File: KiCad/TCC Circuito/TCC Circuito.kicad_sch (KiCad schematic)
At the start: 6 parts, among them J1 Sensor HALL, J2 Rasp pico, U1 TL071, U2 INA333xxDGK, U3 ADS1115IDGS

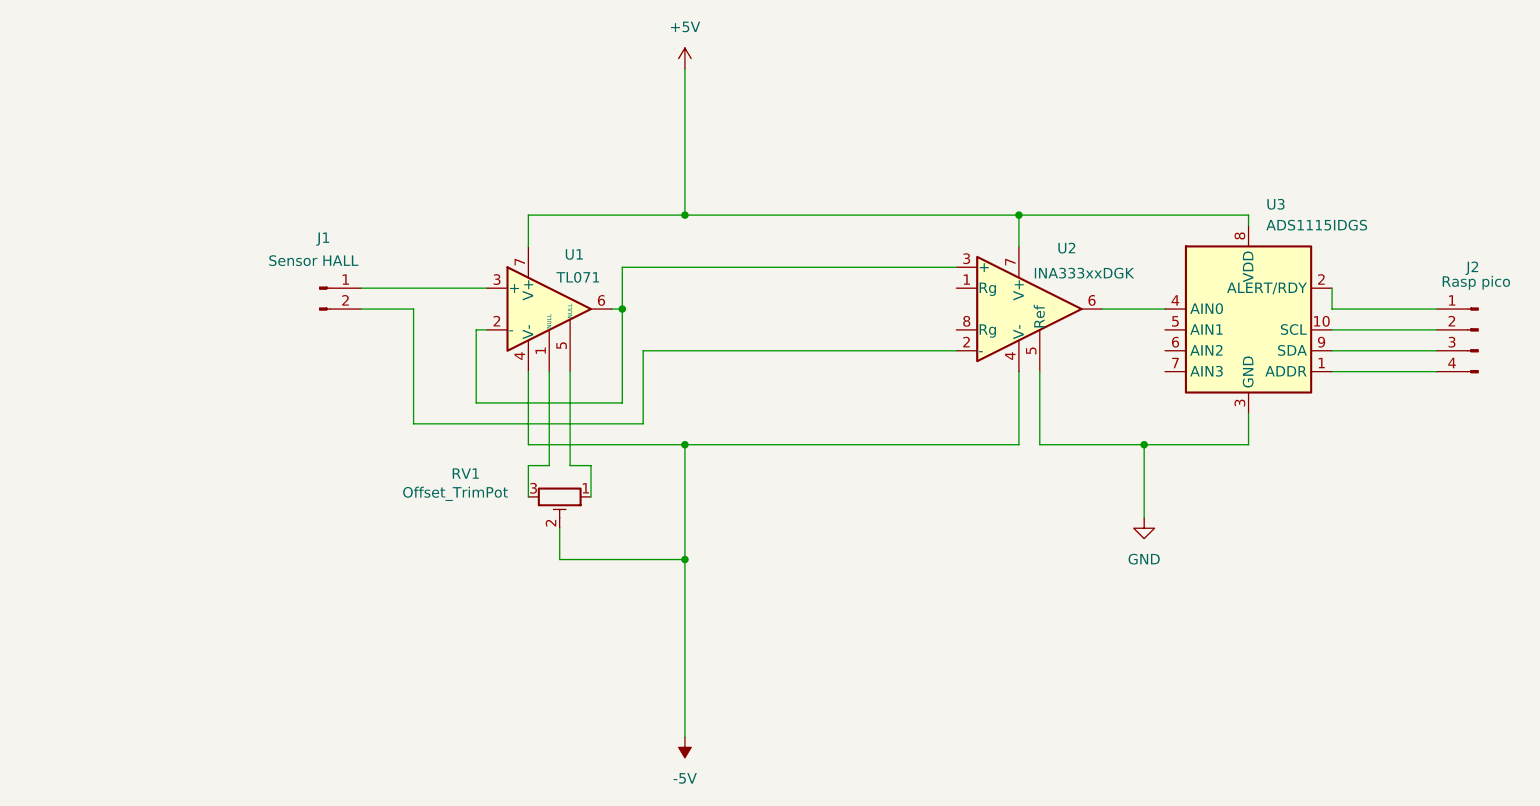
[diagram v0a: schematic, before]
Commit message: dois buffers
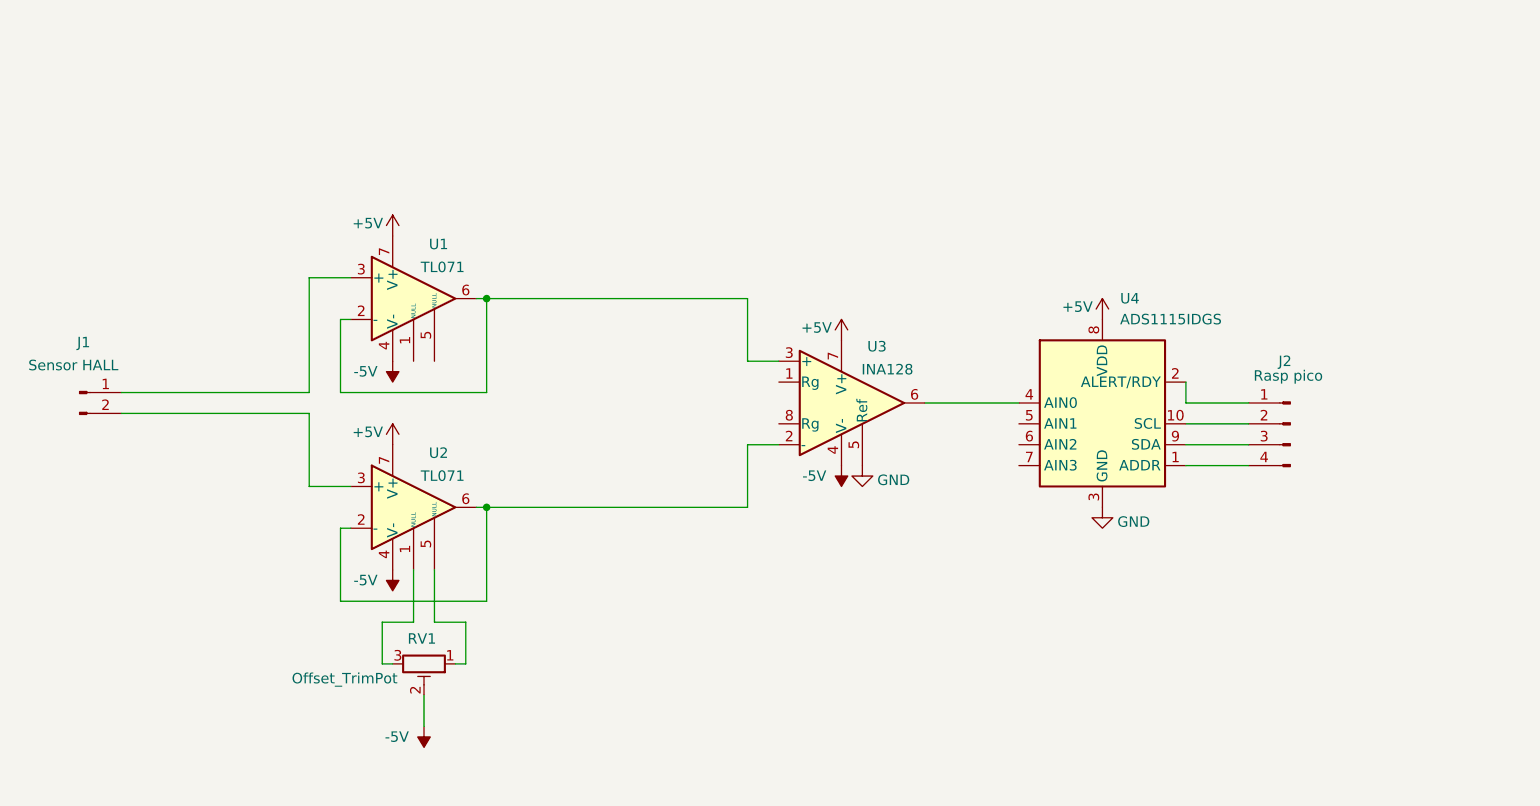
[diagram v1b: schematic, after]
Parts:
- removed U2: INA333xxDGK, Package_SO:VSSOP-8_3x3mm_P0.65mm, symbol Amplifier_Instrumentation:INA333xxDGK
- removed U3: ADS1115IDGS, Package_SO:TSSOP-10_3x3mm_P0.5mm, symbol Analog_ADC:ADS1115IDGS
- added U2: TL071, symbol Amplifier_Operational:TL071
- added U3: INA128, symbol Amplifier_Instrumentation:INA128
- added U4: ADS1115IDGS, Package_SO:TSSOP-10_3x3mm_P0.5mm, symbol Analog_ADC:ADS1115IDGS
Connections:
- net +5V: now also U2.7 (V+), U3.7 (V+), U4.8 (VDD)
- net -5V: now also U2.4 (V-), U3.4 (V-)
- net GND: now also U3.5 (Ref), U4.3 (GND)
- net at J1.2 (Pin_2): now also U2.3 (+)
- net at U1.2 (-), U1.6: now also U3.3 (+)
- net at U1.1 (NULL): no longer RV1.3
- net at U1.5 (NULL): no longer RV1.1
- net at J2.4 (Pin_4): now also U4.1 (ADDR)
- net at J2.2 (Pin_2): now also U4.10 (SCL)
- net at J2.1 (Pin_1): now also U4.2 (ALERT/RDY)
- net at J2.3 (Pin_3): now also U4.9 (SDA)
- new net: RV1.3, U2.1 (NULL)
- new net: U2.2 (-), U2.6, U3.2 (-)
- new net: RV1.1, U2.5 (NULL)
- new net: U3.6, U4.4 (AIN0)
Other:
- moved on the sheet: J1
